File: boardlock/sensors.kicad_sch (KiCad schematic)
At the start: 16 parts, among them Q2 Q_NPN_BCE, Q3 Q_NPN_BCE, Q4 BSS84PWH6327XTSA1, U1 LSM6DSO32, U3 SAM-M8Q

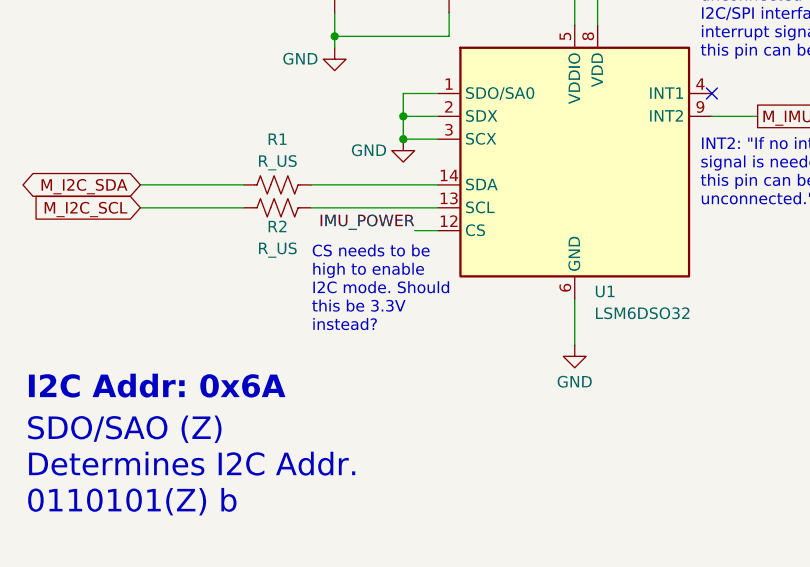
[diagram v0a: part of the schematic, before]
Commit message: modifications?
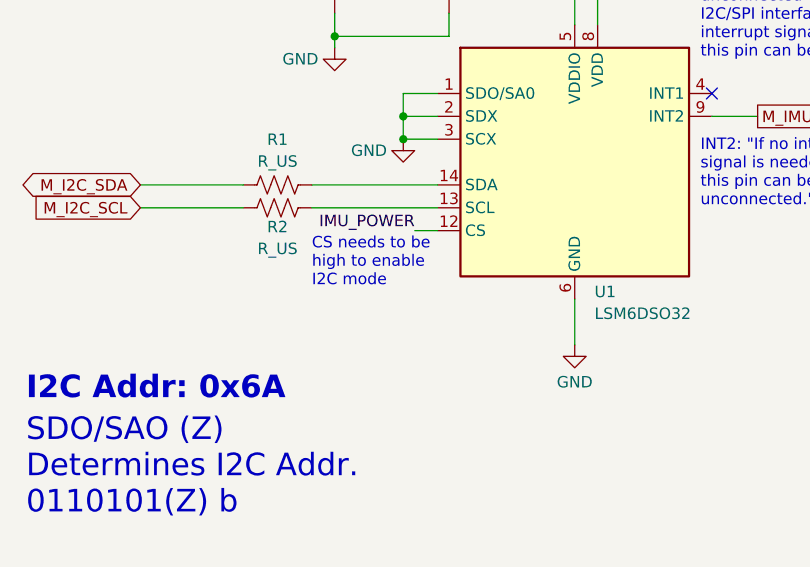
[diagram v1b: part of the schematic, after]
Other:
- note added: "CS needs to be high to enable I2C mode"
- note removed: "CS needs to be high to enable I2C mode. Should this be 3.3V instead?"
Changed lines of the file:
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@@
     (effects (font (size 1.27 1.27)) (justify left bottom))
   )
-  (text "CS needs to be \nhigh to enable \nI2C mode. Should \nthis be 3.3V \ninstead?"
-    (at 59.69 157.48 0)
+  (text "CS needs to be \nhigh to enable \nI2C mode" (at 59.69 152.4 0)
     (effects (font (size 1.27 1.27)) (justify left bottom))
   )
